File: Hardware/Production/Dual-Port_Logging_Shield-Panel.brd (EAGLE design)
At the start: 130 x 203.2 mm, 1821 parts, among them IC1 USB224X_2241_V04, IC10 USB224X_2241_V04, IC11 USB224X_2241_V04, IC12 USB224X_2241_V04, IC13 USB224X_2241_V04, IC14 USB224X_2241_V04, IC15 USB224X_2241_V04, IC2 USB224X_2241_V04, IC3 USB224X_2241_V04, IC4 USB224X_2241_V04, IC5 USB224X_2241_V04, IC6 USB224X_2241_V04, IC7 USB224X_2241_V04, IC8 USB224X_2241_V04, IC9 USB224X_2241_V04, J10 MICRO-SD-PUSH-PUSH-EXT-PIN, J11 AVR_SPI_PROG_3X2TESTPOINTS, J12 THING_PLUS, J14 MICRO-SD-PUSH-PUSH-EXT-PIN, J15 AVR_SPI_PROG_3X2TESTPOINTS, J16 THING_PLUS, J18 MICRO-SD-PUSH-PUSH-EXT-PIN, J19 AVR_SPI_PROG_3X2TESTPOINTS, J2 MICRO-SD-PUSH-PUSH-EXT-PIN, J20 THING_PLUS, J22 MICRO-SD-PUSH-PUSH-EXT-PIN, J23 AVR_SPI_PROG_3X2TESTPOINTS, J24 THING_PLUS, J26 MICRO-SD-PUSH-PUSH-EXT-PIN, J27 AVR_SPI_PROG_3X2TESTPOINTS, J28 THING_PLUS, J3 AVR_SPI_PROG_3X2TESTPOINTS, J30 MICRO-SD-PUSH-PUSH-EXT-PIN, J31 AVR_SPI_PROG_3X2TESTPOINTS, J32 THING_PLUS, J34 MICRO-SD-PUSH-PUSH-EXT-PIN, J35 AVR_SPI_PROG_3X2TESTPOINTS, J36 THING_PLUS, J38 MICRO-SD-PUSH-PUSH-EXT-PIN, J39 AVR_SPI_PROG_3X2TESTPOINTS, J4 THING_PLUS, J40 THING_PLUS, J42 MICRO-SD-PUSH-PUSH-EXT-PIN, J43 AVR_SPI_PROG_3X2TESTPOINTS, J44 THING_PLUS, J46 MICRO-SD-PUSH-PUSH-EXT-PIN, J47 AVR_SPI_PROG_3X2TESTPOINTS, J48 THING_PLUS, J50 MICRO-SD-PUSH-PUSH-EXT-PIN, J51 AVR_SPI_PROG_3X2TESTPOINTS, J52 THING_PLUS, J54 MICRO-SD-PUSH-PUSH-EXT-PIN, J55 AVR_SPI_PROG_3X2TESTPOINTS, J56 THING_PLUS, J58 MICRO-SD-PUSH-PUSH-EXT-PIN, J59 AVR_SPI_PROG_3X2TESTPOINTS, J6 MICRO-SD-PUSH-PUSH-EXT-PIN, J60 THING_PLUS, J7 AVR_SPI_PROG_3X2TESTPOINTS, J8 THING_PLUS, Q1 20V/4.2A/52mΩ/1.4W, Q10 20V/0.2A/8MHz/1.2Ω/1Vth, Q100 20V/4.2A/52mΩ/1.4W, Q101 20V/0.2A/8MHz/1.2Ω/1Vth, Q102 20V/4.2A/52mΩ/1.4W, Q104 20V/4.2A/52mΩ/1.4W, Q11 20V/4.2A/52mΩ/1.4W, Q13 20V/4.2A/52mΩ/1.4W, Q15 20V/4.2A/52mΩ/1.4W, Q16 20V/4.2A/52mΩ/1.4W, Q17 20V/0.2A/8MHz/1.2Ω/1Vth, Q18 20V/4.2A/52mΩ/1.4W, Q2 20V/0.2A/8MHz/1.2Ω/1Vth, Q20 20V/4.2A/52mΩ/1.4W, Q22 20V/4.2A/52mΩ/1.4W, Q23 20V/4.2A/52mΩ/1.4W, Q24 20V/0.2A/8MHz/1.2Ω/1Vth, Q25 20V/4.2A/52mΩ/1.4W, Q27 20V/4.2A/52mΩ/1.4W, Q29 20V/4.2A/52mΩ/1.4W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

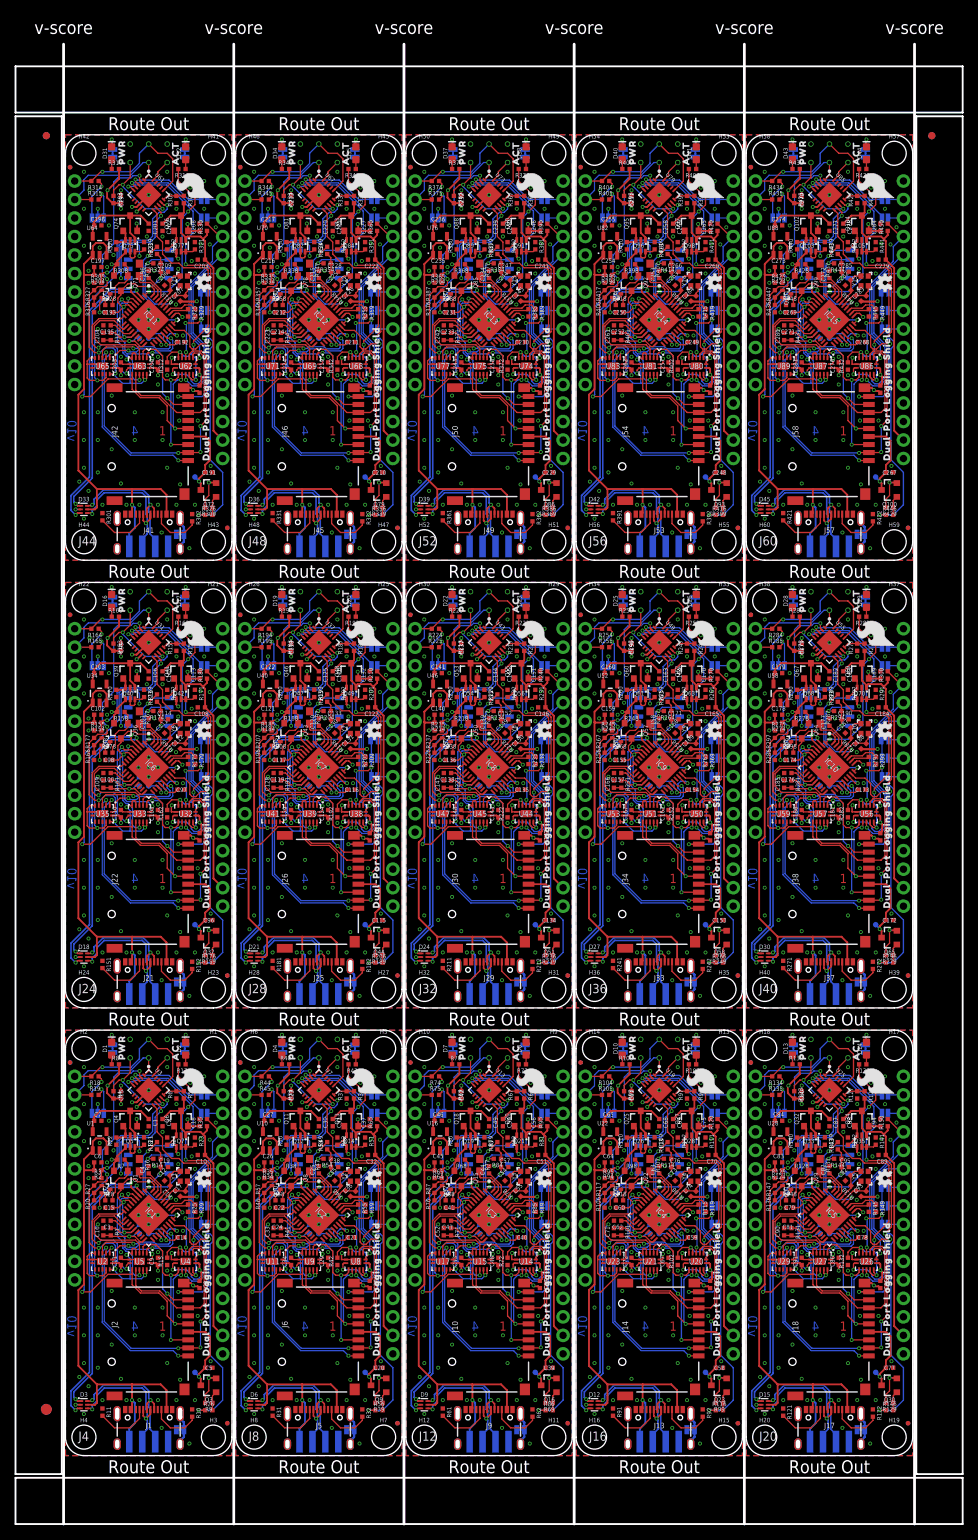
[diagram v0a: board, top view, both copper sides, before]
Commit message: PCB v1.1
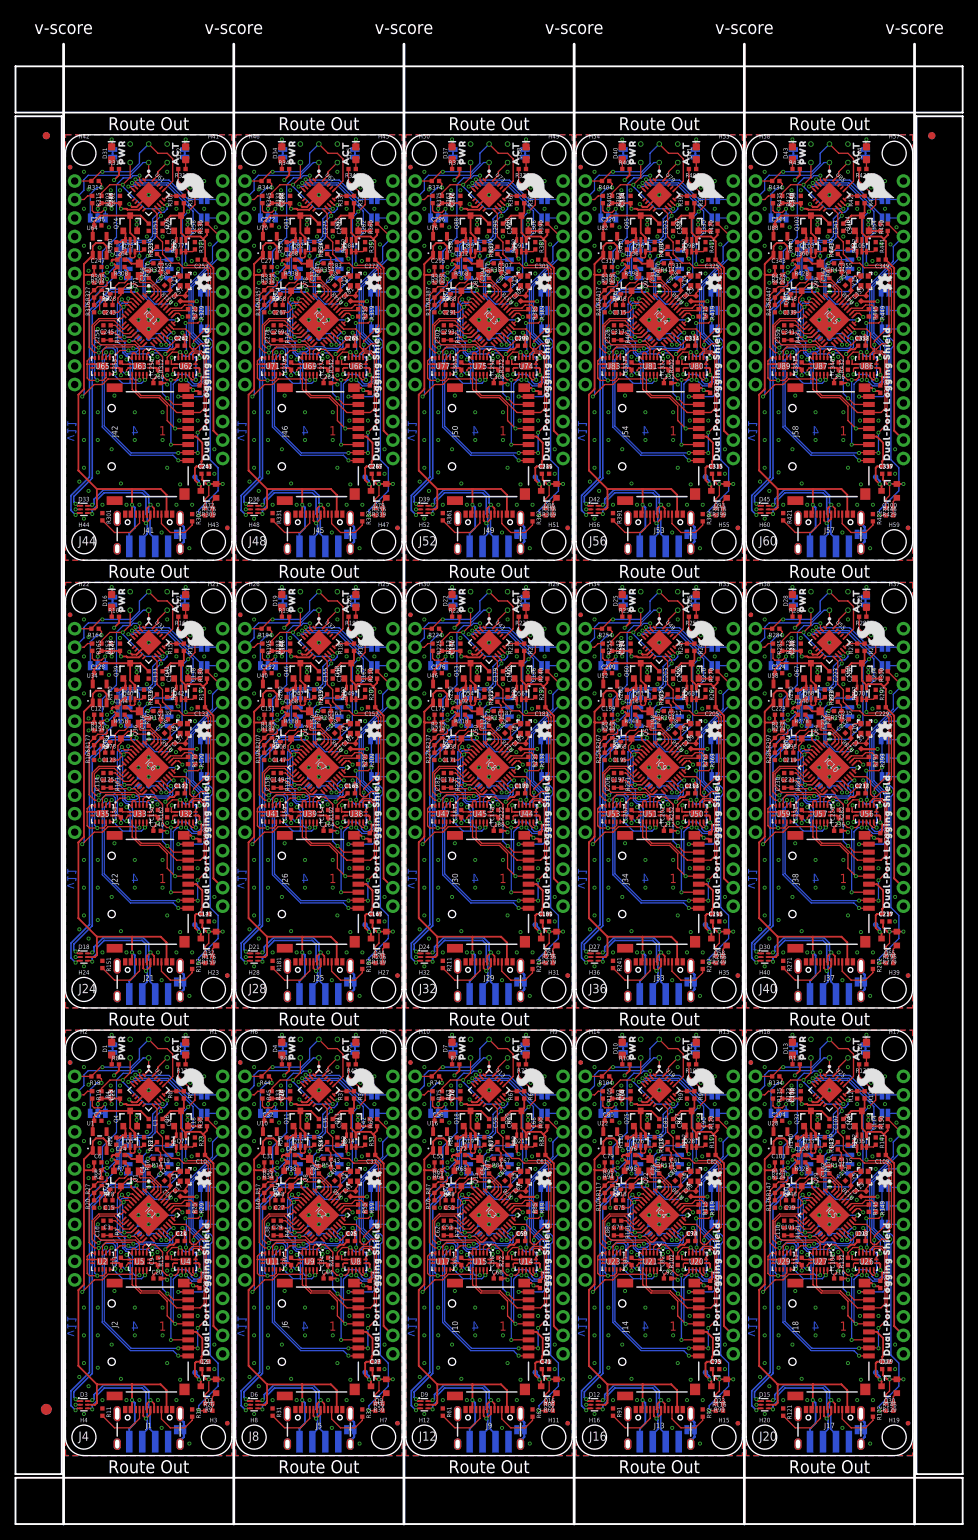
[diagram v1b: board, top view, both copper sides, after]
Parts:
- added C286, C287, C288, C308, C309, C310, C311, C312, C332, C333, C334, C335, C336, C356, C357, C358, C359, C360: 10uF, SparkFun-Capacitors:0402-TIGHT
- added C289, C290, C292, C297, C298, C299, C300, C302, C303, C307, C313, C314, C316, C321, C322, C323, C324, C326, C327, C331, C337, C338, C340, C345, C346, C347, C348, C350, C351, C355: 0.1uF, SparkFun-Capacitors:0402-TIGHT
- added C291, C293, C294, C295, C296, C301, C306, C315, C317, C318, C319, C320, C325, C330, C339, C341, C342, C343, C344, C349, C354: 2.2uF, SparkFun-Capacitors:0402-TIGHT
- added C304, C305, C328, C329, C352, C353: 12pF, SparkFun-Capacitors:0402-TIGHT
- C100, C108, C121, C122, C132, C139, C146, C155, C158, C159, C170, C177, C178, C179, C193, C196, C203, C217, C227, C231, C235, C241, C25, C250, C252, C254, C255, C26, C265, C273, C274, C279, C43, C60, C62, C63, C81, C82, C83, C84, C98: value 2.2uF -> 0.1uF
- C104, C109, C114, C123, C125, C126, C128, C133, C147, C152, C162, C171, C173, C175, C181, C186, C199, C200, C205, C210, C219, C221, C223, C224, C229, C243, C247, C248, C258, C267, C270, C277, C29, C30, C31, C42, C53, C61, C66, C77, C78, C80, C85, C90, C99: value 0.1uF -> 2.2uF
- C111, C130, C131, C169, C187, C206, C207, C225, C226, C244, C283, C35, C36, C73, C74: value 12pF -> 0.1uF
- C113, C136, C160, C184, C208, C233, C41, C64, C65, C89: value 2.2uF -> 12pF
- C116, C118, C142, C143, C144, C164, C166, C167, C190, C191, C192, C20, C21, C213, C23, C237, C238, C239, C240, C261, C262, C285, C47, C48, C68, C69, C71, C72, C95, C96: value 0.1uF -> 10uF
- C117, C119, C120, C140, C141, C165, C189, C212, C214, C215, C216, C22, C236, C24, C260, C284, C44, C45, C46, C70, C94: value 2.2uF -> 10uF
- C137, C161, C185, C209, C232, C256, C257, C280, C281, C40, C88: value 0.1uF -> 12pF
- C149, C150, C245, C282, C54, C55: value 12pF -> 2.2uF
- C168, C188, C263, C264, C92, C93: value 12pF -> 10uF
- I2C, I2C1, I2C10, I2C11, I2C12, I2C13, I2C14, I2C2, I2C3, I2C4, I2C5, I2C6, I2C7, I2C8, I2C9: value JUMPER-SMT_3_NO_SILK -> JUMPER-SMT_3_2-NC_TRACE_SILK; device SparkFun-Jumpers:SMT-JUMPER_3_NO_SILK -> SparkFun-Jumpers:SMT-JUMPER_3_2-NC_TRACE_SILK
- moved C217 127.0 mm to (112.6, 74.4)
- moved C97 124.6 mm to (112.6, 12.9)
- moved C106 124.3 mm to (106.2, 26.7), turned to 90 degrees
- moved C98 122.1 mm to (109.3, 30.5), turned to 0 degrees
- moved C99 119.8 mm to (99.4, 34.0), turned to 180 degrees
- moved C109 118.4 mm to (112.1, 41.3), turned to 180 degrees
- moved C105 118.4 mm to (111.9, 23.5), turned to 270 degrees
- moved C102 118.3 mm to (104.9, 39.2), turned to 90 degrees
- moved C193 117.3 mm to (89.3, 74.4), turned to 0 degrees
- moved C119 117.0 mm to (112.6, 11.9), turned to 0 degrees
- moved C113 115.7 mm to (109.6, 35.9), turned to 45 degrees
- moved C103 115.1 mm to (97.9, 40.3)
- moved C201 113.8 mm to (88.5, 85.0)
- moved C111 113.6 mm to (101.1, 26.7), turned to 90 degrees
- moved C114 112.8 mm to (111.9, 45.7), turned to 90 degrees
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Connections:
- net 3.3V1: now also C36.1, C37.1; no longer C31.1, C32.1
- net 3.3V10: now also C252.1, C253.1; no longer C202.1, C203.1
- net 3.3V11: now also C276.1, C277.1; no longer C221.1, C222.1
- net 3.3V12: now also C300.1, C301.1; no longer C240.1, C241.1
- net 3.3V13: now also C324.1, C325.1; no longer C259.1, C260.1
- net 3.3V14: now also C348.1, C349.1; no longer C278.1, C279.1
- net 3.3V2: now also C60.1, C61.1; no longer C50.1, C51.1
- net 3.3V3: now also C84.1, C85.1; no longer C69.1, C70.1
- net 3.3V4: now also C108.1, C109.1; no longer C88.1, C89.1
- net 3.3V5: now also C132.1, C133.1; no longer C107.1, C108.1
- net 3.3V6: now also C156.1, C157.1; no longer C126.1, C127.1
- net 3.3V7: now also C180.1, C181.1; no longer C145.1, C146.1
- net 3.3V8: now also C204.1, C205.1; no longer C164.1, C165.1
- net 3.3V9: now also C228.1, C229.1; no longer C183.1, C184.1
- net GND: now also C20.2, C21.2, C22.2, C23.2, C24.2
- net GND1: now also C35.2, C36.2, C39.2, C40.1, C41.1, C42.2, C43.2, C44.2, C45.2, C46.2, C47.2, C48.2; no longer C20.2, C21.2, C22.2, C23.2, C24.2, C35.1, C36.1
- net GND10: now also C241.2, C242.2, C243.2, C244.2, C245.2, C246.2, C247.2, C248.2, C249.2, C250.2, C251.2, C252.2, C253.2, C254.2, C255.2, C256.1, C257.1, C258.2, C259.2, C260.2, C261.2, C262.2, C263.2, C264.2; no longer C191.2, C192.2, C193.2, C194.2, C195.2, C196.2, C197.2, C198.2, C199.2, C200.2, C201.2, C202.2, C203.2, C204.2, C205.2, C206.1, C207.1, C208.2, C209.2
- net GND11: now also C265.2, C266.2, C267.2, C268.2, C269.2, C270.2, C271.2, C272.2, C273.2, C274.2, C275.2, C276.2, C277.2, C278.2, C279.2, C280.1, C281.1, C282.2, C283.2, C284.2, C285.2, C286.2, C287.2, C288.2; no longer C210.2, C211.2, C212.2, C213.2, C214.2, C215.2, C216.2, C217.2, C218.2, C219.2, C220.2, C221.2, C222.2, C223.2, C224.2, C225.1, C226.1, C227.2, C228.2
- net GND12: now also C289.2, C290.2, C291.2, C292.2, C293.2, C294.2, C295.2, C296.2, C297.2, C298.2, C299.2, C300.2, C301.2, C302.2, C303.2, C304.1, C305.1, C306.2, C307.2, C308.2, C309.2, C310.2, C311.2, C312.2; no longer C229.2, C230.2, C231.2, C232.2, C233.2, C234.2, C235.2, C236.2, C237.2, C238.2, C239.2, C240.2, C241.2, C242.2, C243.2, C244.1, C245.1, C246.2, C247.2
- net GND13: now also C313.2, C314.2, C315.2, C316.2, C317.2, C318.2, C319.2, C320.2, C321.2, C322.2, C323.2, C324.2, C325.2, C326.2, C327.2, C328.1, C329.1, C330.2, C331.2, C332.2, C333.2, C334.2, C335.2, C336.2; no longer C248.2, C249.2, C250.2, C251.2, C252.2, C253.2, C254.2, C255.2, C256.2, C257.2, C258.2, C259.2, C260.2, C261.2, C262.2, C263.1, C264.1, C265.2, C266.2
- net GND14: now also C337.2, C338.2, C339.2, C340.2, C341.2, C342.2, C343.2, C344.2, C345.2, C346.2, C347.2, C348.2, C349.2, C350.2, C351.2, C352.1, C353.1, C354.2, C355.2, C356.2, C357.2, C358.2, C359.2, C360.2; no longer C267.2, C268.2, C269.2, C270.2, C271.2, C272.2, C273.2, C274.2, C275.2, C276.2, C277.2, C278.2, C279.2, C280.2, C281.2, C282.1, C283.1, C284.2, C285.2
- net GND2: now also C54.2, C55.2, C58.2, C59.2, C60.2, C61.2, C62.2, C63.2, C64.1, C65.1, C66.2, C67.2, C68.2, C69.2, C70.2, C71.2, C72.2; no longer C39.2, C40.2, C41.2, C42.2, C43.2, C44.2, C45.2, C46.2, C47.2, C48.2, C54.1, C55.1
- net GND3: now also C73.2, C74.2, C77.2, C78.2, C79.2, C80.2, C81.2, C82.2, C83.2, C84.2, C85.2, C86.2, C87.2, C88.1, C89.1, C90.2, C91.2, C92.2, C93.2, C94.2, C95.2, C96.2; no longer C58.2, C59.2, C60.2, C61.2, C62.2, C63.2, C64.2, C65.2, C66.2, C67.2, C68.2, C69.2, C70.2, C71.2, C72.2, C73.1, C74.1
- net GND4: now also C100.2, C101.2, C102.2, C103.2, C104.2, C105.2, C106.2, C107.2, C108.2, C109.2, C110.2, C111.2, C112.1, C113.1, C114.2, C115.2, C116.2, C117.2, C118.2, C119.2, C120.2, C97.2, C98.2, C99.2; no longer C77.2, C78.2, C79.2, C80.2, C81.2, C82.2, C83.2, C84.2, C85.2, C86.2, C87.2, C88.2, C89.2, C90.2, C91.2, C92.1, C93.1, C94.2, C95.2
- net GND5: now also C121.2, C122.2, C123.2, C124.2, C125.2, C126.2, C127.2, C128.2, C129.2, C130.2, C131.2, C132.2, C133.2, C134.2, C135.2, C136.1, C137.1, C138.2, C139.2, C140.2, C141.2, C142.2, C143.2, C144.2; no longer C100.2, C101.2, C102.2, C103.2, C104.2, C105.2, C106.2, C107.2, C108.2, C109.2, C110.2, C111.1, C112.1, C113.2, C114.2, C96.2, C97.2, C98.2, C99.2
- net GND6: now also C145.2, C146.2, C147.2, C148.2, C149.2, C150.2, C151.2, C152.2, C153.2, C154.2, C155.2, C156.2, C157.2, C158.2, C159.2, C160.1, C161.1, C162.2, C163.2, C164.2, C165.2, C166.2, C167.2, C168.2; no longer C115.2, C116.2, C117.2, C118.2, C119.2, C120.2, C121.2, C122.2, C123.2, C124.2, C125.2, C126.2, C127.2, C128.2, C129.2, C130.1, C131.1, C132.2, C133.2
- net GND7: now also C169.2, C170.2, C171.2, C172.2, C173.2, C174.2, C175.2, C176.2, C177.2, C178.2, C179.2, C180.2, C181.2, C182.2, C183.2, C184.1, C185.1, C186.2, C187.2, C188.2, C189.2, C190.2, C191.2, C192.2; no longer C134.2, C135.2, C136.2, C137.2, C138.2, C139.2, C140.2, C141.2, C142.2, C143.2, C144.2, C145.2, C146.2, C147.2, C148.2, C149.1, C150.1, C151.2, C152.2
- net GND8: now also C193.2, C194.2, C195.2, C196.2, C197.2, C198.2, C199.2, C200.2, C201.2, C202.2, C203.2, C204.2, C205.2, C206.2, C207.2, C208.1, C209.1, C210.2, C211.2, C212.2, C213.2, C214.2, C215.2, C216.2; no longer C153.2, C154.2, C155.2, C156.2, C157.2, C158.2, C159.2, C160.2, C161.2, C162.2, C163.2, C164.2, C165.2, C166.2, C167.2, C168.1, C169.1, C170.2, C171.2
- net GND9: now also C217.2, C218.2, C219.2, C220.2, C221.2, C222.2, C223.2, C224.2, C225.2, C226.2, C227.2, C228.2, C229.2, C230.2, C231.2, C232.1, C233.1, C234.2, C235.2, C236.2, C237.2, C238.2, C239.2, C240.2; no longer C172.2, C173.2, C174.2, C175.2, C176.2, C177.2, C178.2, C179.2, C180.2, C181.2, C182.2, C183.2, C184.2, C185.2, C186.2, C187.1, C188.1, C189.2, C190.2
- net MICROSD_VCC1: now also C25.1; no longer C20.1
- net MICROSD_VCC10: now also C241.1; no longer C191.1
- net MICROSD_VCC11: now also C265.1; no longer C210.1
- net MICROSD_VCC12: now also C289.1; no longer C229.1
- net MICROSD_VCC13: now also C313.1; no longer C248.1
- net MICROSD_VCC14: now also C337.1; no longer C267.1
- net MICROSD_VCC2: now also C49.1; no longer C39.1
- net MICROSD_VCC3: now also C73.1; no longer C58.1
- net MICROSD_VCC4: now also C97.1; no longer C77.1
- net MICROSD_VCC5: now also C121.1; no longer C96.1
- net MICROSD_VCC6: now also C145.1; no longer C115.1
- net MICROSD_VCC7: now also C169.1; no longer C134.1
- net MICROSD_VCC8: now also C193.1; no longer C153.1
- net MICROSD_VCC9: now also C217.1; no longer C172.1
- net N$116: now also C101.1; no longer C81.1
- net N$117: now also C102.1; no longer C82.1
- net N$142: now also C125.1; no longer C100.1
- net N$143: now also C126.1; no longer C101.1
- net N$168: now also C149.1; no longer C119.1
- net N$169: now also C150.1; no longer C120.1
- net N$194: now also C173.1; no longer C138.1
- net N$195: now also C174.1; no longer C139.1
- net N$220: now also C197.1; no longer C157.1
- net N$221: now also C198.1; no longer C158.1
- net N$246: now also C221.1; no longer C176.1
- net N$247: now also C222.1; no longer C177.1
- net N$272: now also C245.1; no longer C195.1
- net N$273: now also C246.1; no longer C196.1
- net N$298: now also C269.1; no longer C214.1
- net N$299: now also C270.1; no longer C215.1
- net N$324: now also C293.1; no longer C233.1
- net N$325: now also C294.1; no longer C234.1
- net N$350: now also C317.1; no longer C252.1
- net N$351: now also C318.1; no longer C253.1
- net N$376: now also C341.1; no longer C271.1
- net N$377: now also C342.1; no longer C272.1
- net N$38: now also C29.1; no longer C24.1
- net N$39: now also C30.1; no longer C25.1
- net N$64: now also C53.1; no longer C43.1
- net N$65: now also C54.1; no longer C44.1
- net N$90: now also C77.1; no longer C62.1
- net N$91: now also C78.1; no longer C63.1
- net SDIO_!RESET!1: now also C38.1; no longer C33.1
- net SDIO_!RESET!10: now also C254.1; no longer C204.1
- net SDIO_!RESET!11: now also C278.1; no longer C223.1
- net SDIO_!RESET!12: now also C302.1; no longer C242.1
- net SDIO_!RESET!13: now also C326.1; no longer C261.1
- net SDIO_!RESET!14: now also C350.1; no longer C280.1
- net SDIO_!RESET!2: now also C62.1; no longer C52.1
- net SDIO_!RESET!3: now also C86.1; no longer C71.1
- net SDIO_!RESET!4: now also C110.1; no longer C90.1
- net SDIO_!RESET!5: now also C134.1; no longer C109.1
- net SDIO_!RESET!6: now also C158.1; no longer C128.1
- net SDIO_!RESET!7: now also C182.1; no longer C147.1
- net SDIO_!RESET!8: now also C206.1; no longer C166.1
- net SDIO_!RESET!9: now also C230.1; no longer C185.1
- net SDIO_VDD1: now also C26.1, C27.1, C43.1; no longer C21.1, C22.1, C38.1
- net SDIO_VDD10: now also C242.1, C243.1, C259.1; no longer C192.1, C193.1, C209.1
- net SDIO_VDD11: now also C266.1, C267.1, C283.1; no longer C211.1, C212.1, C228.1
- net SDIO_VDD12: now also C290.1, C291.1, C307.1; no longer C230.1, C231.1, C247.1
- net SDIO_VDD13: now also C314.1, C315.1, C331.1; no longer C249.1, C250.1, C266.1
- net SDIO_VDD14: now also C338.1, C339.1, C355.1; no longer C268.1, C269.1, C285.1
- net SDIO_VDD2: now also C50.1, C51.1, C67.1; no longer C40.1, C41.1, C57.1
- net SDIO_VDD3: now also C74.1, C75.1, C91.1; no longer C59.1, C60.1, C76.1
- net SDIO_VDD4: now also C115.1, C98.1, C99.1; no longer C78.1, C79.1, C95.1
- net SDIO_VDD5: now also C122.1, C123.1, C139.1; no longer C114.1, C97.1, C98.1
- net SDIO_VDD6: now also C146.1, C147.1, C163.1; no longer C116.1, C117.1, C133.1
- net SDIO_VDD7: now also C170.1, C171.1, C187.1; no longer C135.1, C136.1, C152.1
- net SDIO_VDD8: now also C194.1, C195.1, C211.1; no longer C154.1, C155.1, C171.1
- net SDIO_VDD9: now also C218.1, C219.1, C235.1; no longer C173.1, C174.1, C190.1
- net VCC: now also C20.1, C21.1, C22.1, C23.1, C24.1
- net VCC1: now also C33.1, C39.1, C42.1, C44.1, C45.1, C46.1, C47.1, C48.1; no longer C23.1, C29.1, C37.1
- net VCC10: now also C244.1, C249.1, C250.1, C255.1, C258.1, C260.1, C261.1, C262.1, C263.1, C264.1; no longer C194.1, C199.1, C200.1, C205.1, C208.1
- net VCC11: now also C268.1, C273.1, C274.1, C279.1, C282.1, C284.1, C285.1, C286.1, C287.1, C288.1; no longer C213.1, C218.1, C219.1, C224.1, C227.1
- net VCC12: now also C292.1, C297.1, C298.1, C303.1, C306.1, C308.1, C309.1, C310.1, C311.1, C312.1; no longer C232.1, C237.1, C238.1, C243.1, C246.1
- net VCC13: now also C316.1, C321.1, C322.1, C327.1, C330.1, C332.1, C333.1, C334.1, C335.1, C336.1; no longer C251.1, C256.1, C257.1, C262.1, C265.1
- net VCC14: now also C340.1, C345.1, C346.1, C351.1, C354.1, C356.1, C357.1, C358.1, C359.1, C360.1; no longer C270.1, C275.1, C276.1, C281.1, C284.1
- net VCC2: now also C52.1, C57.1, C58.1, C63.1, C66.1, C68.1, C69.1, C70.1, C71.1, C72.1; no longer C42.1, C47.1, C48.1, C53.1, C56.1
- net VCC3: now also C76.1, C81.1, C82.1, C87.1, C90.1, C92.1, C93.1, C94.1, C95.1, C96.1; no longer C61.1, C66.1, C67.1, C72.1, C75.1
- net VCC4: now also C100.1, C105.1, C106.1, C111.1, C114.1, C116.1, C117.1, C118.1, C119.1, C120.1; no longer C80.1, C85.1, C86.1, C91.1, C94.1
- net VCC5: now also C124.1, C129.1, C130.1, C135.1, C138.1, C140.1, C141.1, C142.1, C143.1, C144.1; no longer C104.1, C105.1, C110.1, C113.1, C99.1
- net VCC6: now also C148.1, C153.1, C154.1, C159.1, C162.1, C164.1, C165.1, C166.1, C167.1, C168.1; no longer C118.1, C123.1, C124.1, C129.1, C132.1
- net VCC7: now also C172.1, C177.1, C178.1, C183.1, C186.1, C188.1, C189.1, C190.1, C191.1, C192.1; no longer C137.1, C142.1, C143.1, C148.1, C151.1
- net VCC8: now also C196.1, C201.1, C202.1, C207.1, C210.1, C212.1, C213.1, C214.1, C215.1, C216.1; no longer C156.1, C161.1, C162.1, C167.1, C170.1
- net VCC9: now also C220.1, C225.1, C226.1, C231.1, C234.1, C236.1, C237.1, C238.1, C239.1, C240.1; no longer C175.1, C180.1, C181.1, C186.1, C189.1
- net VCC_10: now also C224.1, C227.1; no longer C179.1, C182.1
- net VCC_11: now also C248.1, C251.1; no longer C198.1, C201.1
- net VCC_12: now also C272.1, C275.1; no longer C217.1, C220.1
- net VCC_13: now also C296.1, C299.1; no longer C236.1, C239.1
- net VCC_14: now also C320.1, C323.1; no longer C255.1, C258.1
- net VCC_15: now also C344.1, C347.1; no longer C274.1, C277.1
- net VCC_2: now also C32.1, C35.1; no longer C27.1, C30.1
- net VCC_3: now also C56.1, C59.1; no longer C46.1, C49.1
- net VCC_4: now also C80.1, C83.1; no longer C65.1, C68.1
- net VCC_5: now also C104.1, C107.1; no longer C84.1, C87.1
- net VCC_6: now also C128.1, C131.1; no longer C103.1, C106.1
- net VCC_7: now also C152.1, C155.1; no longer C122.1, C125.1
- net VCC_8: now also C176.1, C179.1; no longer C141.1, C144.1
- net VCC_9: now also C200.1, C203.1; no longer C160.1, C163.1
- net V_USB1: now also C31.1; no longer C26.1
- net V_USB10: now also C247.1; no longer C197.1
- net V_USB11: now also C271.1; no longer C216.1
- net V_USB12: now also C295.1; no longer C235.1
- net V_USB13: now also C319.1; no longer C254.1
- net V_USB14: now also C343.1; no longer C273.1
- net V_USB2: now also C55.1; no longer C45.1
- net V_USB3: now also C79.1; no longer C64.1
- net V_USB4: now also C103.1; no longer C83.1
- net V_USB5: now also C127.1; no longer C102.1
- net V_USB6: now also C151.1; no longer C121.1
- net V_USB7: now also C175.1; no longer C140.1
- net V_USB8: now also C199.1; no longer C159.1
- net V_USB9: now also C223.1; no longer C178.1
- net XTAL10: now also C112.2; no longer C92.2
- net XTAL11: now also C137.2; no longer C112.2
- net XTAL12: now also C136.2; no longer C111.2
- net XTAL13: now also C161.2; no longer C131.2
- net XTAL14: now also C160.2; no longer C130.2
- net XTAL15: now also C185.2; no longer C150.2
- net XTAL16: now also C184.2; no longer C149.2
- net XTAL17: now also C209.2; no longer C169.2
- net XTAL18: now also C208.2; no longer C168.2
- net XTAL19: now also C233.2; no longer C188.2
- net XTAL20: now also C232.2; no longer C187.2
- net XTAL21: now also C257.2; no longer C207.2
- net XTAL22: now also C256.2; no longer C206.2
- net XTAL23: now also C281.2; no longer C226.2
- net XTAL24: now also C280.2; no longer C225.2
- net XTAL25: now also C305.2; no longer C245.2
- net XTAL26: now also C304.2; no longer C244.2
- net XTAL27: now also C329.2; no longer C264.2
- net XTAL28: now also C328.2; no longer C263.2
- net XTAL29: now also C353.2; no longer C283.2
- net XTAL3: now also C41.2; no longer C36.2
- net XTAL30: now also C352.2; no longer C282.2
- net XTAL4: now also C40.2; no longer C35.2
- net XTAL5: now also C65.2; no longer C55.2
- net XTAL6: now also C64.2; no longer C54.2
- net XTAL7: now also C89.2; no longer C74.2
- net XTAL8: now also C88.2; no longer C73.2
- net XTAL9: now also C113.2; no longer C93.2
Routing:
- net VCC10: track 31.1 -> 40.6 mm, vias 12 -> 16
- net VCC14: track 31.1 -> 40.6 mm, vias 12 -> 16
- net VCC12: track 31.1 -> 40.6 mm, vias 12 -> 16
- net VCC11: track 31.1 -> 40.6 mm, vias 12 -> 16
- net VCC4: track 31.1 -> 40.6 mm, vias 12 -> 16
- net VCC: track 31.1 -> 40.6 mm, vias 12 -> 16
- net VCC13: track 31.1 -> 40.6 mm, vias 12 -> 16
- net VCC9: track 31.1 -> 40.6 mm, vias 12 -> 16
- net VCC2: track 31.1 -> 40.6 mm, vias 12 -> 16
- net VCC3: track 31.1 -> 40.6 mm, vias 12 -> 16
- net VCC7: track 31.1 -> 40.6 mm, vias 12 -> 16
- net VCC5: track 31.1 -> 40.6 mm, vias 12 -> 16
- net VCC1: track 31.1 -> 40.6 mm, vias 12 -> 16
- net VCC6: track 31.1 -> 40.6 mm, vias 12 -> 16
- net VCC8: track 31.1 -> 40.6 mm, vias 12 -> 16
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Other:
- board text added: "v11"
- board text removed: "v10"
